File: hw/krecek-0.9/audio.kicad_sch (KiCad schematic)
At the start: 6 parts, among them CN1 PJ-313B6-B, U10 TPA2028D1YZFT, U11 ES8312

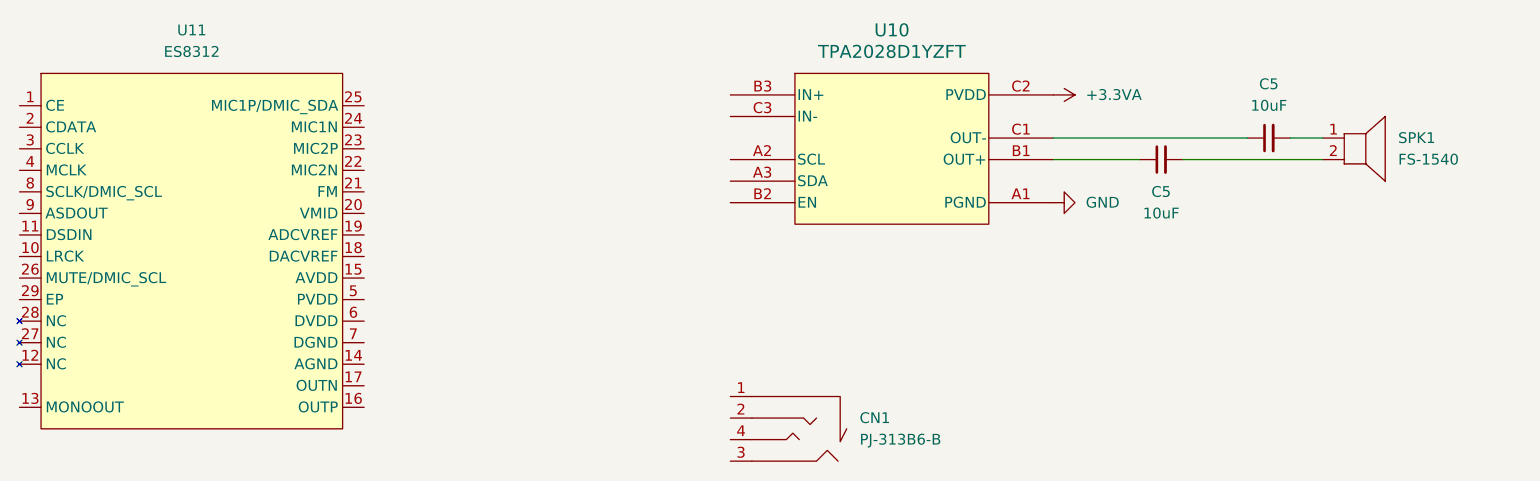
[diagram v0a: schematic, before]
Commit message: Fix amplifier/speaker connection
Signed-off-by: Jan Hamal Dvořák <mordae@anilinux.org>
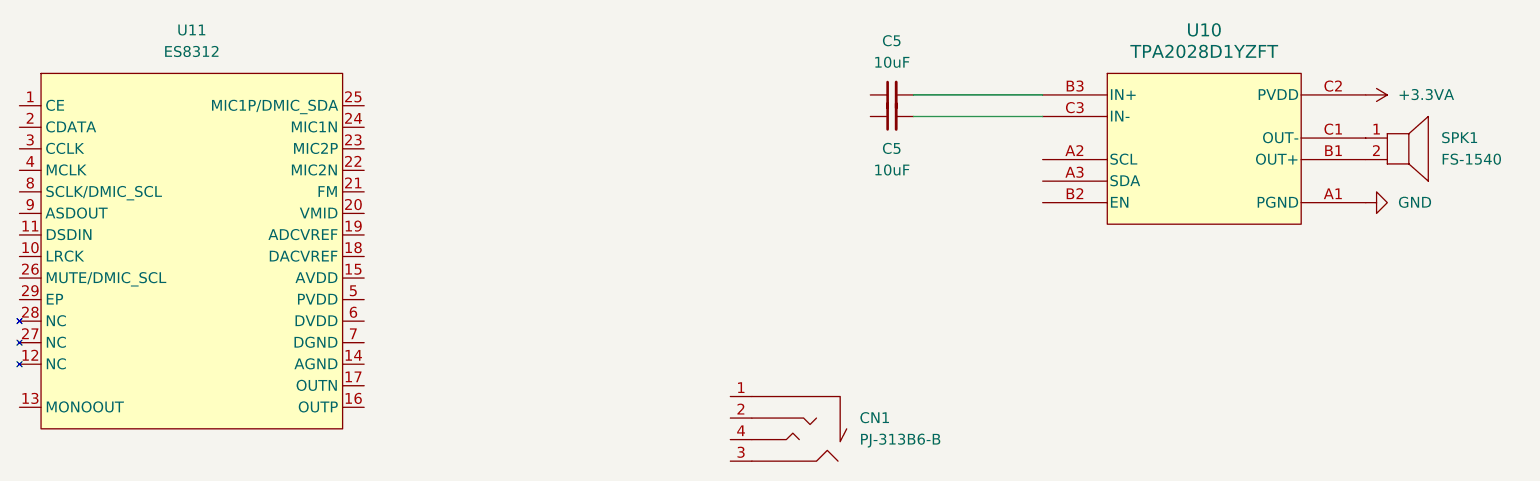
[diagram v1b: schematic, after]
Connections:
- net at SPK1.1 (+): now also U10.C1 (OUT-); no longer C5.2
- net at SPK1.2: now also U10.B1 (OUT+); no longer C5.2
- net at C5.1: no longer U10.B1 (OUT+)
- net at U10.B3 (IN+): now also C5.2
- net at C5.1: no longer U10.C1 (OUT-)
- net at U10.C3 (IN-): now also C5.2
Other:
- moved on the sheet: C5, SPK1, U10
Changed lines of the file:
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@@
 (kicad_sch (version 20230121) (generator eeschema)
   (paper "A4")
-  (wire (pts (xy 222.25 60.96) (xy 232.41 60.96))
+  (wire (pts (xy 205.74 55.88) (xy 220.98 55.88))
     (stroke (width 0) (type default))
   )
-  (wire (pts (xy 250.19 58.42) (xy 254 58.42))
+  (wire (pts (xy 205.74 53.34) (xy 220.98 53.34))
     (stroke (width 0) (type default))
   )
-  (wire (pts (xy 237.49 60.96) (xy 254 60.96))
-    (stroke (width 0) (type default))
-  )
-  (wire (pts (xy 222.25 58.42) (xy 245.11 58.42))
-    (stroke (width 0) (type default))
-  )
-  (symbol (lib_id "power:GND") (at 222.25 66.04 90) (unit 1)
-    (in_bom yes) (on_board yes) (dnp no) (fields_autoplaced)
-    (property "Reference" "#PWR031" (at 228.6 66.04 0)
-      (effects (font (size 1.27 1.27)) hide)
-    )
-    (property "Value" "GND" (at 226.06 66.04 90)
+  (symbol (lib_id "power:GND") (at 259.08 66.04 90) (unit 1)
+    (in_bom yes) (on_board yes) (dnp no) (fields_autoplaced)
+    (property "Reference" "#PWR031" (at 265.43 66.04 0)
+      (effects (font (size 1.27 1.27)) hide)
+    )
+    (property "Value" "GND" (at 262.89 66.04 90)
       (effects (font (size 1.27 1.27)) (justify right))
     )
-    (property "Footprint" "" (at 222.25 66.04 0)
-      (effects (font (size 1.27 1.27)) hide)
-    )
-    (property "Datasheet" "" (at 222.25 66.04 0)
+    (property "Footprint" "" (at 259.08 66.04 0)
+      (effects (font (size 1.27 1.27)) hide)
+    )
+    (property "Datasheet" "" (at 259.08 66.04 0)
       (effects (font (size 1.27 1.27)) hide)
     )
@@
     )
   )
-  (symbol (lib_id "LCSC:FS-1540") (at 257.81 59.69 0) (unit 1)
-    (in_bom yes) (on_board yes) (dnp no) (fields_autoplaced)
-    (property "Reference" "SPK1" (at 262.89 58.42 0)
+  (symbol (lib_id "LCSC:FS-1540") (at 262.89 59.69 0) (unit 1)
+    (in_bom yes) (on_board yes) (dnp no) (fields_autoplaced)
+    (property "Reference" "SPK1" (at 267.97 58.42 0)
       (effects (font (size 1.27 1.27)) (justify left))
     )
-    (property "Value" "FS-1540" (at 262.89 60.96 0)
+    (property "Value" "FS-1540" (at 267.97 60.96 0)
       (effects (font (size 1.27 1.27)) (justify left))
     )
-    (property "Footprint" "LCSC:BUZ-SMD_5P-L15.0-W15.0-P13.7-BL" (at 257.81 72.39 0)
-      (effects (font (size 1.27 1.27)) hide)
-    )
-    (property "Datasheet" "" (at 257.81 59.69 0)
-      (effects (font (size 1.27 1.27)) hide)
-    )
-    (property "LCSC Part" "C482341" (at 257.81 74.93 0)
+    (property "Footprint" "LCSC:BUZ-SMD_5P-L15.0-W15.0-P13.7-BL" (at 262.89 72.39 0)
+      (effects (font (size 1.27 1.27)) hide)
+    )
+    (property "Datasheet" "" (at 262.89 59.69 0)
+      (effects (font (size 1.27 1.27)) hide)
+    )
+    (property "LCSC Part" "C482341" (at 262.89 74.93 0)
       (effects (font (size 1.27 1.27)) hide)
     )
@@
     )
   )
-  (symbol (lib_id "LCSC:TPA2028D1YZFT") (at 203.2 60.96 0) (unit 1)
-    (in_bom yes) (on_board yes) (dnp no) (fields_autoplaced)
-    (property "Reference" "U10" (at 203.2 45.72 0)
+  (symbol (lib_id "LCSC:TPA2028D1YZFT") (at 240.03 60.96 0) (unit 1)
+    (in_bom yes) (on_board yes) (dnp no) (fields_autoplaced)
+    (property "Reference" "U10" (at 240.03 45.72 0)
       (effects (font (size 1.524 1.524)))
     )
-    (property "Value" "TPA2028D1YZFT" (at 203.2 48.26 0)
+    (property "Value" "TPA2028D1YZFT" (at 240.03 48.26 0)
       (effects (font (size 1.524 1.524)))
     )
-    (property "Footprint" "LCSC:TPA2028" (at 203.2 73.66 0)
+    (property "Footprint" "LCSC:TPA2028" (at 240.03 73.66 0)
       (effects (font (size 1.27 1.27) italic) hide)
     )
-    (property "Datasheet" "TPA2028D1YZFT" (at 203.2 76.2 0)
+    (property "Datasheet" "TPA2028D1YZFT" (at 240.03 76.2 0)
       (effects (font (size 1.27 1.27) italic) hide)
     )
@@
     )
   )
-  (symbol (lib_id "Device:C_Small") (at 234.95 60.96 90) (mirror x) (unit 1)
-    (in_bom yes) (on_board yes) (dnp no) (fields_autoplaced)
-    (property "Reference" "C5" (at 234.9563 64.77 90)
-      (effects (font (size 1.27 1.27)))
-    )
-    (property "Value" "10uF" (at 234.9563 67.31 90)
-      (effects (font (size 1.27 1.27)))
-    )
-    (property "Footprint" "Capacitor_SMD:C_0805_2012Metric" (at 234.95 60.96 0)
-      (effects (font (size 1.27 1.27)) hide)
-    )
-    (property "Datasheet" "~" (at 234.95 60.96 0)
-      (effects (font (size 1.27 1.27)) hide)
-    )
-    (property "LCSC Part" "C15850" (at 234.95 60.96 0)
+  (symbol (lib_id "Device:C_Small") (at 203.2 55.88 90) (mirror x) (unit 1)
+    (in_bom yes) (on_board yes) (dnp no) (fields_autoplaced)
+    (property "Reference" "C5" (at 203.2063 59.69 90)
+      (effects (font (size 1.27 1.27)))
+    )
+    (property "Value" "10uF" (at 203.2063 62.23 90)
+      (effects (font (size 1.27 1.27)))
+    )
+    (property "Footprint" "Capacitor_SMD:C_0805_2012Metric" (at 203.2 55.88 0)
+      (effects (font (size 1.27 1.27)) hide)
+    )
+    (property "Datasheet" "~" (at 203.2 55.88 0)
+      (effects (font (size 1.27 1.27)) hide)
+    )
+    (property "LCSC Part" "C15850" (at 203.2 55.88 0)
       (effects (font (size 1.27 1.27)) hide)
     )
@@
     )
   )
-  (symbol (lib_id "power:+3.3VA") (at 222.25 53.34 270) (unit 1)
-    (in_bom yes) (on_board yes) (dnp no) (fields_autoplaced)
-    (property "Reference" "#PWR032" (at 218.44 53.34 0)
-      (effects (font (size 1.27 1.27)) hide)
-    )
-    (property "Value" "+3.3VA" (at 226.06 53.34 90)
+  (symbol (lib_id "power:+3.3VA") (at 259.08 53.34 270) (unit 1)
+    (in_bom yes) (on_board yes) (dnp no) (fields_autoplaced)
+    (property "Reference" "#PWR032" (at 255.27 53.34 0)
+      (effects (font (size 1.27 1.27)) hide)
+    )
+    (property "Value" "+3.3VA" (at 262.89 53.34 90)
       (effects (font (size 1.27 1.27)) (justify left))
     )
-    (property "Footprint" "" (at 222.25 53.34 0)
-      (effects (font (size 1.27 1.27)) hide)
-    )
-    (property "Datasheet" "" (at 222.25 53.34 0)
+    (property "Footprint" "" (at 259.08 53.34 0)
+      (effects (font (size 1.27 1.27)) hide)
+    )
+    (property "Datasheet" "" (at 259.08 53.34 0)
       (effects (font (size 1.27 1.27)) hide)
     )
@@
     )
   )
-  (symbol (lib_id "Device:C_Small") (at 247.65 58.42 90) (unit 1)
-    (in_bom yes) (on_board yes) (dnp no) (fields_autoplaced)
-    (property "Reference" "C5" (at 247.6563 52.07 90)
-      (effects (font (size 1.27 1.27)))
-    )
-    (property "Value" "10uF" (at 247.6563 54.61 90)
-      (effects (font (size 1.27 1.27)))
-    )
-    (property "Footprint" "Capacitor_SMD:C_0805_2012Metric" (at 247.65 58.42 0)
-      (effects (font (size 1.27 1.27)) hide)
-    )
-    (property "Datasheet" "~" (at 247.65 58.42 0)
-      (effects (font (size 1.27 1.27)) hide)
-    )
-    (property "LCSC Part" "C15850" (at 247.65 58.42 0)
-      (effects (font (size 1.27 1.27)) hide)
-    )
+  (symbol (lib_id "Device:C_Small") (at 203.2 53.34 90) (unit 1)
+    (in_bom yes) (on_board yes) (dnp no) (fields_autoplaced)
+    (property "Reference" "C5" (at 203.2063 46.99 90)
+      (effects (font (size 1.27 1.27)))
+    )
+    (property "Value" "10uF" (at 203.2063 49.53 90)
+      (effects (font (size 1.27 1.27)))
+    )
+    (property "Footprint" "Capacitor_SMD:C_0805_2012Metric" (at 203.2 53.34 0)
+      (effects (font (size 1.27 1.27)) hide)
+    )
+    (property "Datasheet" "~" (at 203.2 53.34 0)
+      (effects (font (size 1.27 1.27)) hide)
+    )
+    (property "LCSC Part" "C15850" (at 203.2 53.34 0)
+      (effects (font (size 1.27 1.27)) hide)
+    )
